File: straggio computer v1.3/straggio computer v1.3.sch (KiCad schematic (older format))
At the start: 0 parts

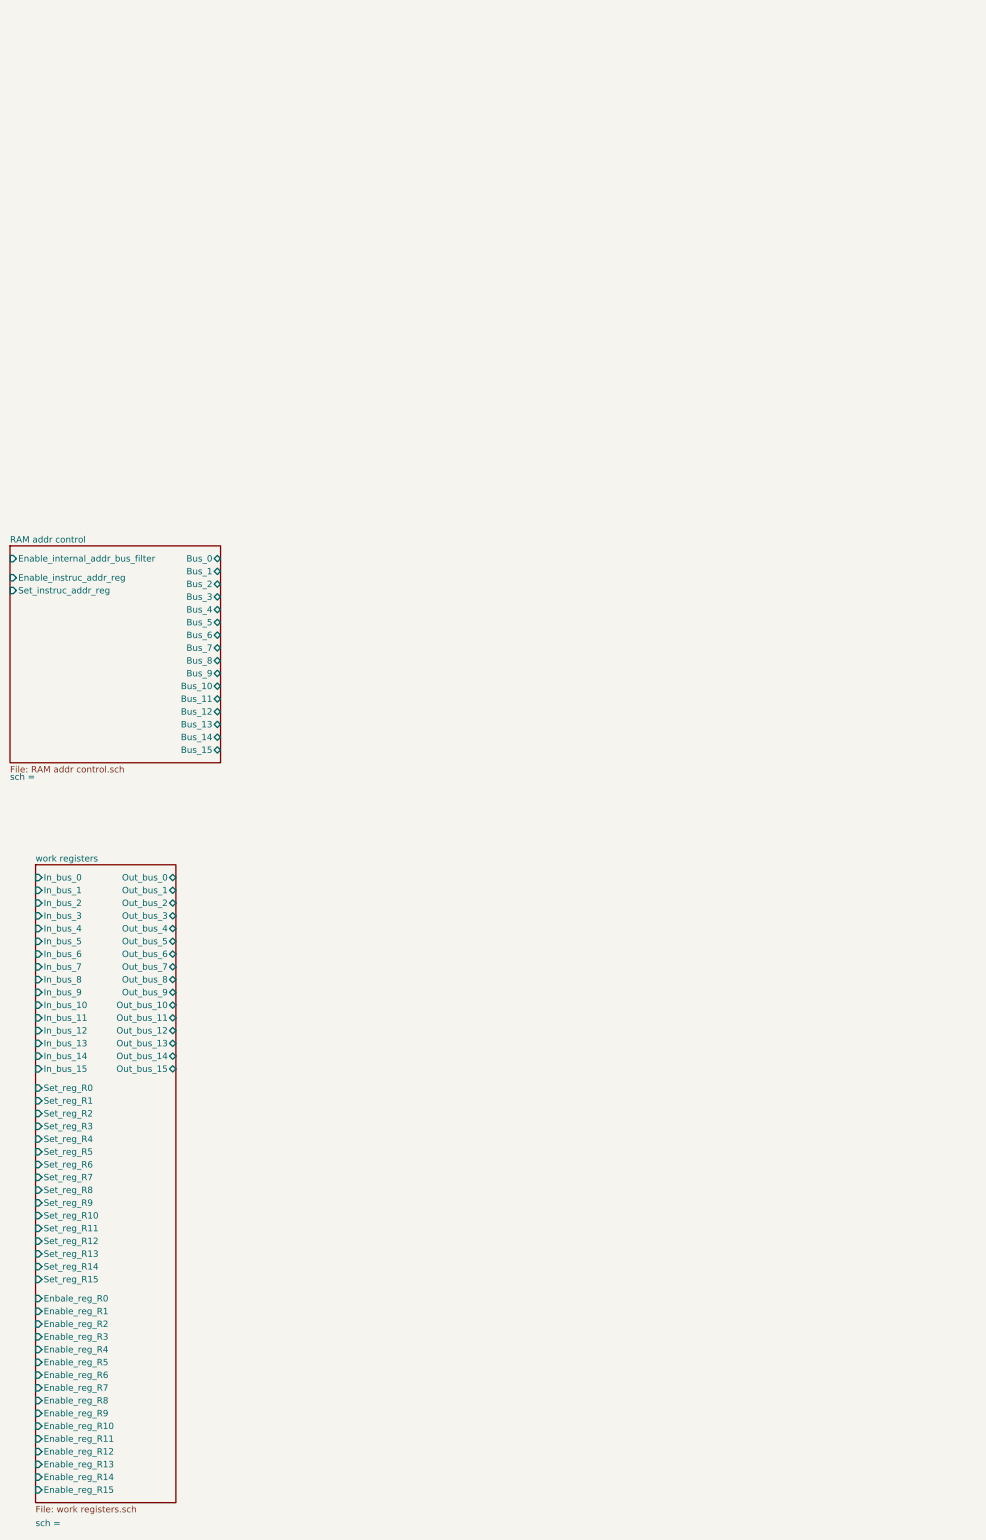
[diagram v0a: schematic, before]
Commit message: Update 24/02/2021
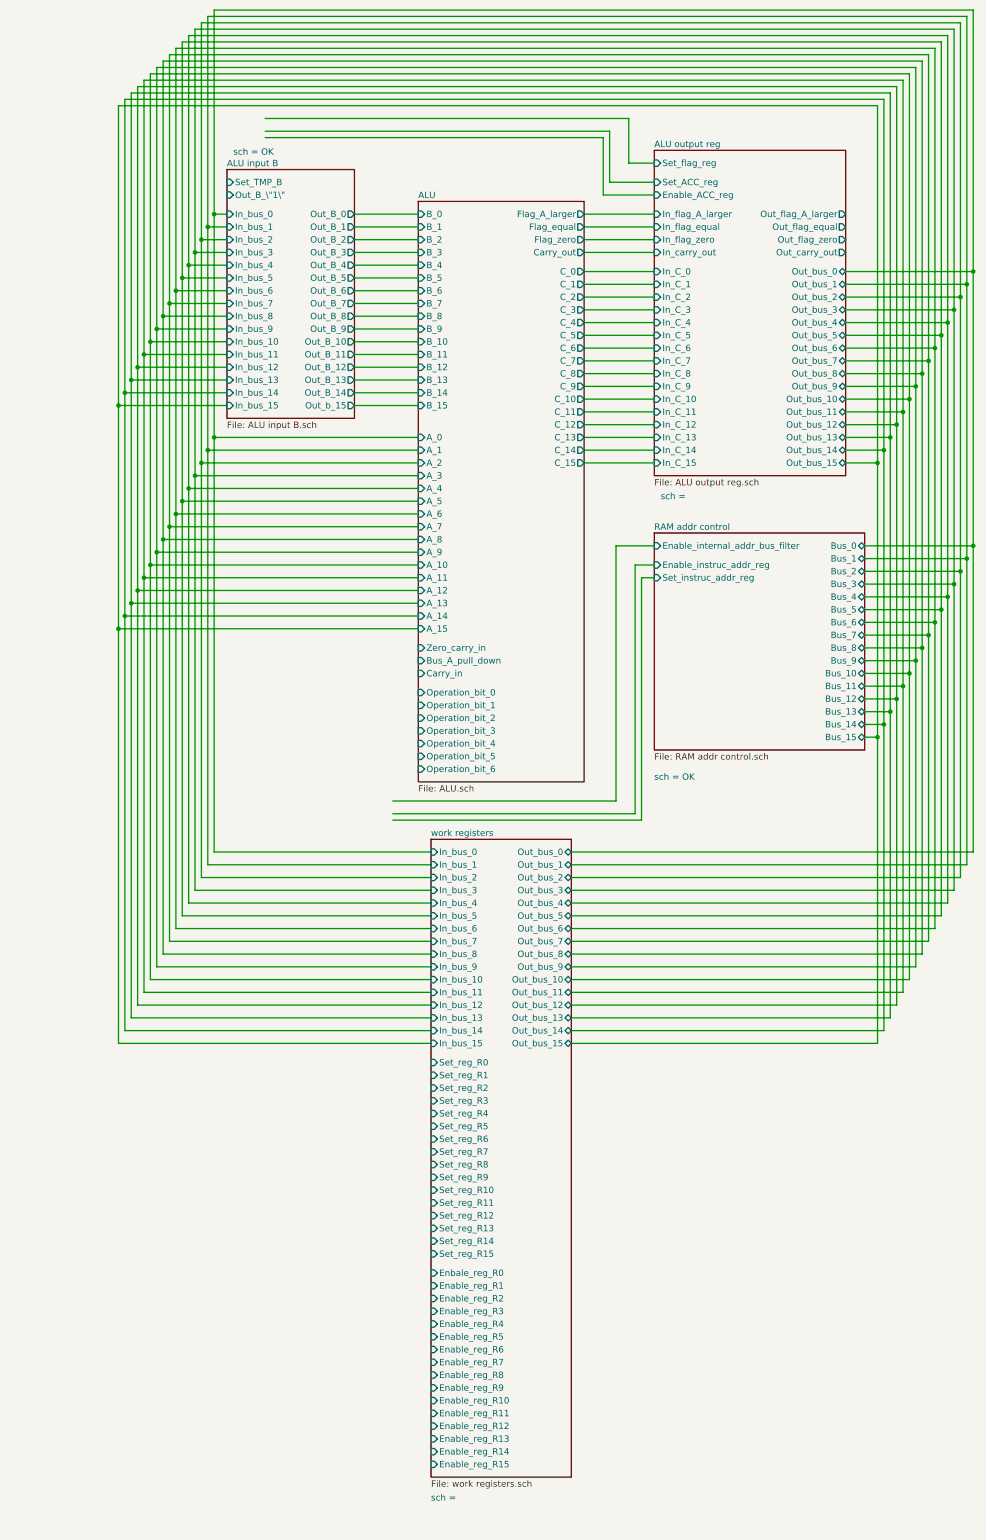
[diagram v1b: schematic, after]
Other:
- note added: "sch = OK"
